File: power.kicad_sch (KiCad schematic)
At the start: 108 parts, among them U41 TPS7A8801RTJR, U42 TPS7A8801RTJR, U43 TPS61252DSG, U44 TPSM863252RDXR, U45 TPS7A3301RGW, U46 TPSM863252RDXR

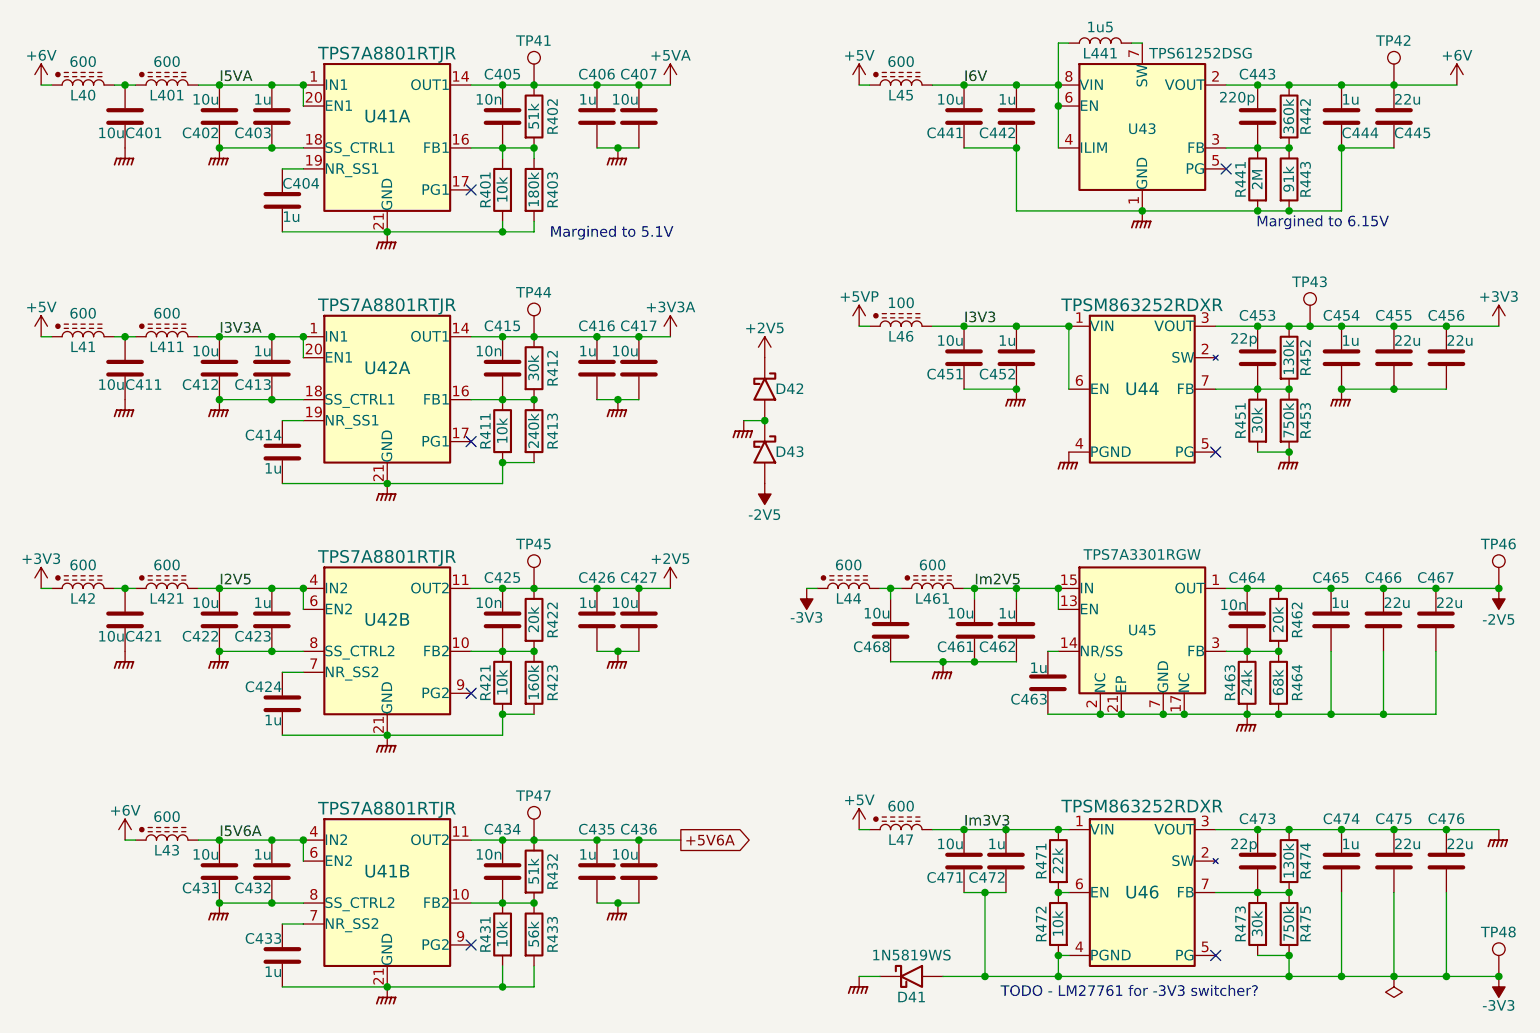
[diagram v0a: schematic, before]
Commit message: Progress checkin.  About to redo FDA feedback again.
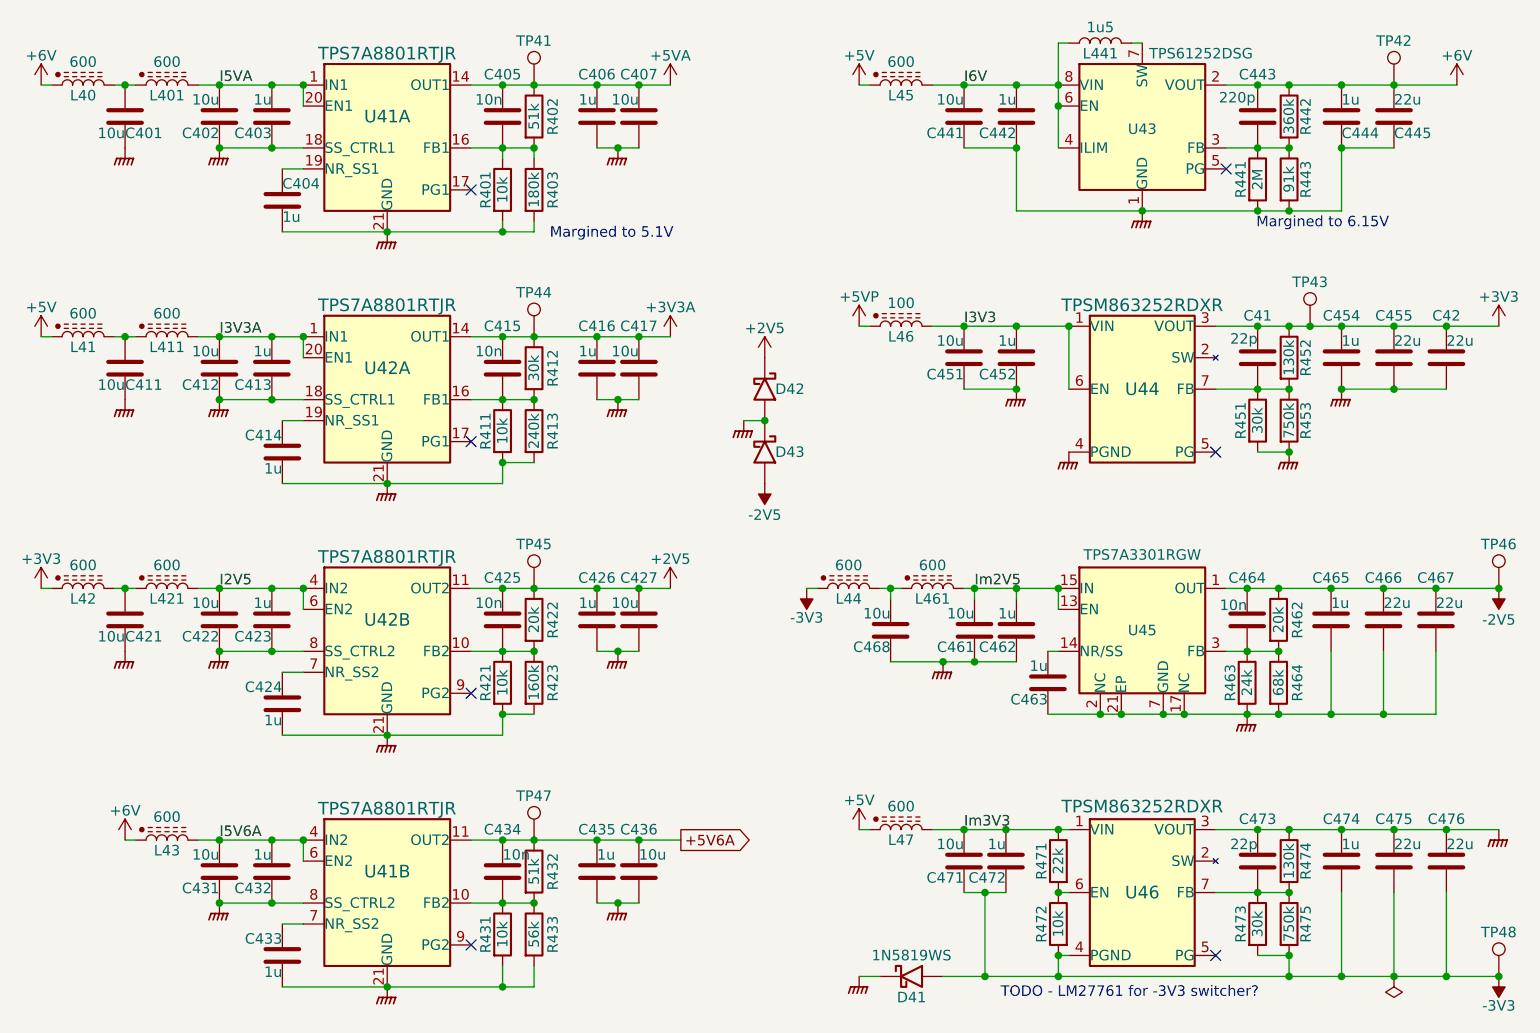
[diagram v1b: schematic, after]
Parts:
- renumbered C453 to C41, C456 to C42
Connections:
- net -2V5: now also C465.1; no longer C465.2
- net GNDPWR: now also C463.2, C465.2; no longer C463.1, C465.1
- net at U45.14 (NR/SS): now also C463.1; no longer C463.2
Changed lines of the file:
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@@
 		(lib_id "Device:C")
 		(at 110.49 137.16 0)
-		(mirror y)
 		(unit 1)
 		(exclude_from_sim no)
@@
 		)
 		(property "Footprint" "Capacitor_SMD:C_0402_1005Metric"
-			(at 109.5248 140.97 0)
+			(at 111.4552 140.97 0)
 			(effects
 				(font
@@
 		(lib_id "Device:R")
 		(at 99.06 83.82 0)
-		(mirror y)
 		(unit 1)
 		(exclude_from_sim no)
@@
 		)
 		(property "Footprint" "Resistor_SMD:R_0402_1005Metric"
-			(at 100.838 83.82 90)
+			(at 97.282 83.82 90)
 			(effects
 				(font
@@
 		(lib_id "Device:C")
 		(at 115.57 137.16 0)
-		(mirror y)
 		(unit 1)
 		(exclude_from_sim no)
@@
 		)
 		(property "Footprint" "Capacitor_SMD:C_0603_1608Metric"
-			(at 114.6048 140.97 0)
+			(at 116.5352 140.97 0)
 			(effects
 				(font
@@
 		(lib_id "Device:R")
 		(at 190.5 53.34 0)
-		(mirror y)
 		(unit 1)
 		(exclude_from_sim no)
@@
 		)
 		(property "Footprint" "Resistor_SMD:R_0603_1608Metric"
-			(at 192.278 53.34 90)
+			(at 188.722 53.34 90)
 			(effects
 				(font
@@
 		(lib_id "Device:R")
 		(at 99.06 144.78 0)
-		(mirror y)
 		(unit 1)
 		(exclude_from_sim no)
@@
 		)
 		(property "Footprint" "Resistor_SMD:R_0402_1005Metric"
-			(at 100.838 144.78 90)
+			(at 97.282 144.78 90)
 			(effects
 				(font
@@
 		(lib_id "Device:R")
 		(at 190.5 143.51 0)
-		(mirror y)
 		(unit 1)
 		(exclude_from_sim no)
@@
 		)
 		(property "Footprint" "Resistor_SMD:R_0603_1608Metric"
-			(at 192.278 143.51 90)
+			(at 188.722 143.51 90)
 			(effects
 				(font
@@
 		(lib_id "Device:C")
 		(at 199.39 106.68 0)
-		(mirror x)
 		(unit 1)
 		(exclude_from_sim no)
@@
 		)
 		(property "Footprint" "Capacitor_SMD:C_0402_1005Metric"
-			(at 200.3552 102.87 0)
+			(at 200.3552 110.49 0)
 			(effects
 				(font
@@
 		(lib_id "Device:C")
 		(at 99.06 137.16 0)
-		(mirror y)
 		(unit 1)
 		(exclude_from_sim no)
@@
 		)
 		(property "Footprint" "Capacitor_SMD:C_0603_1608Metric"
-			(at 98.0948 140.97 0)
+			(at 100.0252 140.97 0)
 			(effects
 				(font
@@
 		(lib_id "Device:R")
 		(at 99.06 114.3 0)
-		(mirror y)
 		(unit 1)
 		(exclude_from_sim no)
@@
 		)
 		(property "Footprint" "Resistor_SMD:R_0402_1005Metric"
-			(at 100.838 114.3 90)
+			(at 97.282 114.3 90)
 			(effects
 				(font
@@
 		(on_board yes)
 		(dnp no)
-		(property "Reference" "C453"
+		(property "Reference" "C41"
 			(at 190.5 69.85 0)
 			(effects
@@
 			(project "lincal"
 				(path "/b054cef4-39e3-49d8-aff0-7ba5a206c187/98a8b958-69ae-452b-9f02-aef214a697d8"
-					(reference "C453")
+					(reference "C41")
 					(unit 1)
 				)
@@
 		(lib_id "Device:C")
 		(at 165.1 114.3 0)
-		(mirror x)
 		(unit 1)
 		(exclude_from_sim no)
@@
 		)
 		(property "Value" "1u"
-			(at 165.1 112.522 0)
+			(at 165.1 112.268 0)
 			(effects
 				(font
@@
 		)
 		(property "Footprint" "Capacitor_SMD:C_0402_1005Metric"
-			(at 166.0652 110.49 0)
+			(at 166.0652 118.11 0)
 			(effects
 				(font
@@
 		(on_board yes)
 		(dnp no)
-		(property "Reference" "C456"
+		(property "Reference" "C42"
 			(at 213.36 69.85 0)
 			(effects
@@
 			(project "lincal"
 				(path "/b054cef4-39e3-49d8-aff0-7ba5a206c187/98a8b958-69ae-452b-9f02-aef214a697d8"
-					(reference "C456")
+					(reference "C42")
 					(unit 1)
 				)
@@
 		(lib_id "Device:R")
 		(at 99.06 54.61 0)
-		(mirror y)
 		(unit 1)
 		(exclude_from_sim no)
@@
 		)
 		(property "Footprint" "Resistor_SMD:R_0402_1005Metric"
-			(at 100.838 54.61 90)
+			(at 97.282 54.61 90)
 			(effects
 				(font
@@
 		(lib_id "Device:R")
 		(at 190.5 82.55 0)
-		(mirror y)
 		(unit 1)
 		(exclude_from_sim no)
@@
 		)
 		(property "Footprint" "Resistor_SMD:R_0603_1608Metric"
-			(at 192.278 82.55 90)
+			(at 188.722 82.55 90)
 			(effects
 				(font
